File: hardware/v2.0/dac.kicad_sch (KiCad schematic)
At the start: 4 parts, among them IC3 LTC2630ISC6-LZ12#TRMPBF, J8 530480210, U1 ECP5U-25F-CABGA256

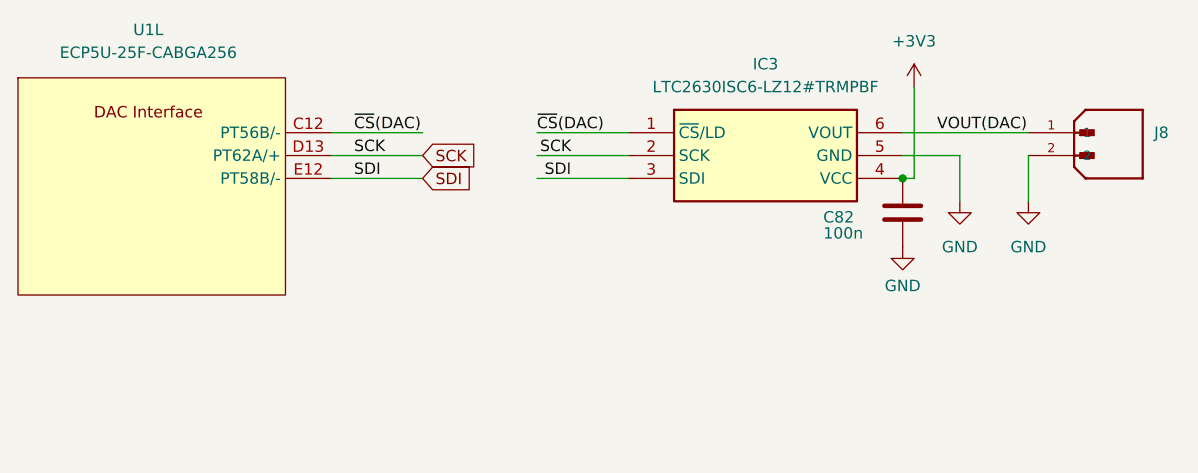
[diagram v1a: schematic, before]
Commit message: ERC pass
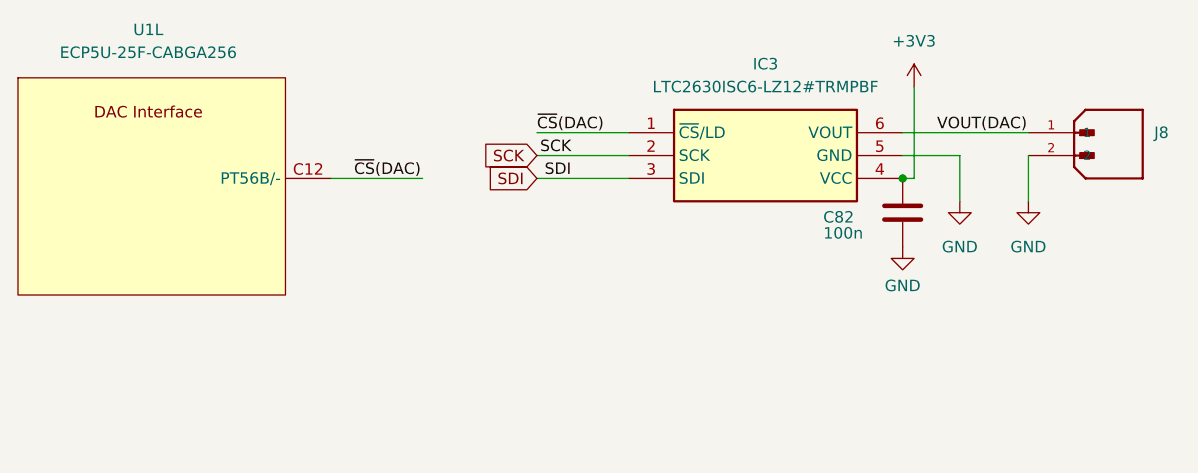
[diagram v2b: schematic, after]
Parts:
- IC3: MANUFACTURER (none) -> ADI; MANUFACTURER_PART_NUMBER (none) -> LTC2630ISC6-LZ12#TRMPBF
- J8: MANUFACTURER_PART_NUMBER (none) -> 0530480210
- U1: MANUFACTURER (none) -> Lattice; MANUFACTURER_PART_NUMBER (none) -> LFE5U-25F-6BG256C
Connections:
- net SCK: no longer U1.D13 (PT62A/+)
- net SDI: no longer U1.E12 (PT58B/-)
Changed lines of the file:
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@@
+	(wire
+		(pts
+			(xy 148.59 95.25) (xy 158.75 95.25)
+		)
+		(stroke
+			(width 0)
+			(type default)
+		)
+	)
+	(wire
+		(pts
+			(xy 148.59 97.79) (xy 158.75 97.79)
+		)
+		(stroke
+			(width 0)
+			(type default)
+		)
+	)
+	(wire
+		(pts
+			(xy 189.23 97.79) (xy 190.5 97.79)
+		)
+		(stroke
+			(width 0)
+			(type default)
+		)
+	)
+	(wire
+		(pts
+			(xy 189.23 92.71) (xy 203.2 92.71)
+		)
+		(stroke
+			(width 0)
+			(type default)
+		)
+	)
+	(wire
+		(pts
+			(xy 203.2 100.33) (xy 203.2 95.25)
+		)
+		(stroke
+			(width 0)
+			(type default)
+		)
+	)
+	(wire
+		(pts
+			(xy 148.59 92.71) (xy 158.75 92.71)
+		)
+		(stroke
+			(width 0)
+			(type default)
+		)
+	)
 	(wire
 		(pts
@@
 	(wire
 		(pts
-			(xy 125.73 95.25) (xy 135.89 95.25)
+			(xy 195.58 95.25) (xy 195.58 100.33)
 		)
 		(stroke
@@
 	(wire
 		(pts
-			(xy 148.59 95.25) (xy 158.75 95.25)
+			(xy 189.23 95.25) (xy 195.58 95.25)
 		)
 		(stroke
 			(width 0)
 			(type default)
-		)
-	)
-	(wire
-		(pts
-			(xy 148.59 97.79) (xy 158.75 97.79)
-		)
-		(stroke
-			(width 0)
-			(type default)
-		)
-	)
-	(wire
-		(pts
-			(xy 189.23 97.79) (xy 190.5 97.79)
-		)
-		(stroke
-			(width 0)
-			(type default)
-		)
-	)
-	(wire
-		(pts
-			(xy 189.23 92.71) (xy 203.2 92.71)
-		)
-		(stroke
-			(width 0)
-			(type default)
-		)
-	)
-	(wire
-		(pts
-			(xy 203.2 100.33) (xy 203.2 95.25)
-		)
-		(stroke
-			(width 0)
-			(type default)
-		)
-	)
-	(wire
-		(pts
-			(xy 148.59 92.71) (xy 158.75 92.71)
-		)
-		(stroke
-			(width 0)
-			(type default)
-		)
-	)
-	(wire
-		(pts
-			(xy 125.73 92.71) (xy 135.89 92.71)
-		)
-		(stroke
-			(width 0)
-			(type default)
-		)
-	)
-	(wire
-		(pts
-			(xy 195.58 95.25) (xy 195.58 100.33)
-		)
-		(stroke
-			(width 0)
-			(type default)
-		)
-	)
-	(wire
-		(pts
-			(xy 189.23 95.25) (xy 195.58 95.25)
-		)
-		(stroke
-			(width 0)
-			(type default)
-		)
-	)
-	(label "SDI"
-		(at 128.27 97.79 0)
-		(effects
-			(font
-				(size 1.27 1.27)
-			)
-			(justify left bottom)
 		)
 	)
@@
 	)
 	(label "~{CS}(DAC)"
-		(at 128.27 92.71 0)
+		(at 128.27 97.79 0)
 		(effects
 			(font
@@
 		)
 	)
-	(label "SCK"
-		(at 128.27 95.25 0)
-		(effects
-			(font
-				(size 1.27 1.27)
-			)
-			(justify left bottom)
-		)
-	)
 	(label "SDI"
 		(at 152.4 97.79 180)
@@
 	(global_label "SCK"
 		(shape input)
-		(at 135.89 95.25 0)
+		(at 148.59 95.25 180)
 		(fields_autoplaced yes)
 		(effects
@@
 				(size 1.27 1.27)
 			)
-			(justify left)
+			(justify right)
 		)
 		(property "Intersheetrefs" "${INTERSHEET_REFS}"
-			(at 142.6247 95.25 0)
-			(effects
-				(font
-					(size 1.27 1.27)
-				)
-				(justify left)
+			(at 141.8553 95.25 0)
+			(effects
+				(font
+					(size 1.27 1.27)
+				)
+				(justify right)
 				(hide yes)
 			)
@@
 	(global_label "SDI"
 		(shape input)
-		(at 135.89 97.79 0)
+		(at 148.59 97.79 180)
 		(fields_autoplaced yes)
 		(effects
@@
 				(size 1.27 1.27)
 			)
-			(justify left)
+			(justify right)
 		)
 		(property "Intersheetrefs" "${INTERSHEET_REFS}"
-			(at 141.9595 97.79 0)
-			(effects
-				(font
-					(size 1.27 1.27)
-				)
-				(justify left)
+			(at 142.5205 97.79 0)
+			(effects
+				(font
+					(size 1.27 1.27)
+				)
+				(justify right)
 				(hide yes)
 			)
@@
 			)
 		)
+		(property "MANUFACTURER" "ADI"
+			(at 158.75 92.71 0)
+			(effects
+				(font
+					(size 1.27 1.27)
+				)
+				(hide yes)
+			)
+		)
+		(property "MANUFACTURER_PART_NUMBER" "LTC2630ISC6-LZ12#TRMPBF"
+			(at 158.75 92.71 0)
+			(effects
+				(font
+					(size 1.27 1.27)
+				)
+				(hide yes)
+			)
+		)
 		(pin "6"
 		)
@@
 			)
 		)
-		(property "Description" ""
+		(property "Description" "Connector Header Through Hole, Right Angle 2 position 0.049\" (1.25mm)"
 			(at 208.28 92.71 0)
 			(effects
@@
 				)
 				(justify bottom)
+				(hide yes)
+			)
+		)
+		(property "MANUFACTURER_PART_NUMBER" "0530480210"
+			(at 208.28 92.71 0)
+			(effects
+				(font
+					(size 1.27 1.27)
+				)
 				(hide yes)
 			)
@@
 			)
 		)
+		(property "MANUFACTURER" "Lattice"
+			(at 105.41 110.49 0)
+			(effects
+				(font
+					(size 1.27 1.27)
+				)
+				(hide yes)
+			)
+		)
+		(property "MANUFACTURER_PART_NUMBER" "LFE5U-25F-6BG256C"
+			(at 105.41 110.49 0)
+			(effects
+				(font
+					(size 1.27 1.27)
+				)
+				(hide yes)
+			)
+		)
 		(pin "M5"
 		)
@@
 		(pin "D13"
 		)
+		(pin "P2"
+		)
+		(pin "P1"
+		)
+		(pin "G13"
+		)
+		(pin "E15"
+		)
+		(pin "N1"
+		)
 		(pin "E12"
 		)
-		(pin "D13"
-		)
-		(pin "P2"
-		)
-		(pin "P1"
-		)
-		(pin "G13"
-		)
-		(pin "E15"
-		)
-		(pin "N1"
-		)
-		(pin "E12"
-		)
 		(pin "G12"
 		)
@@
 		(pin "P4"
 		)
-		(pin "N6"
-		)
 		(pin "K5"
